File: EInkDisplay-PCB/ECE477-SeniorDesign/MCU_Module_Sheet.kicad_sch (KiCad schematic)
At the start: 26 parts, among them J7 Conn_01x05, SW1 SW_Push_Dual_x2, U3 STM32L496ZGTxP

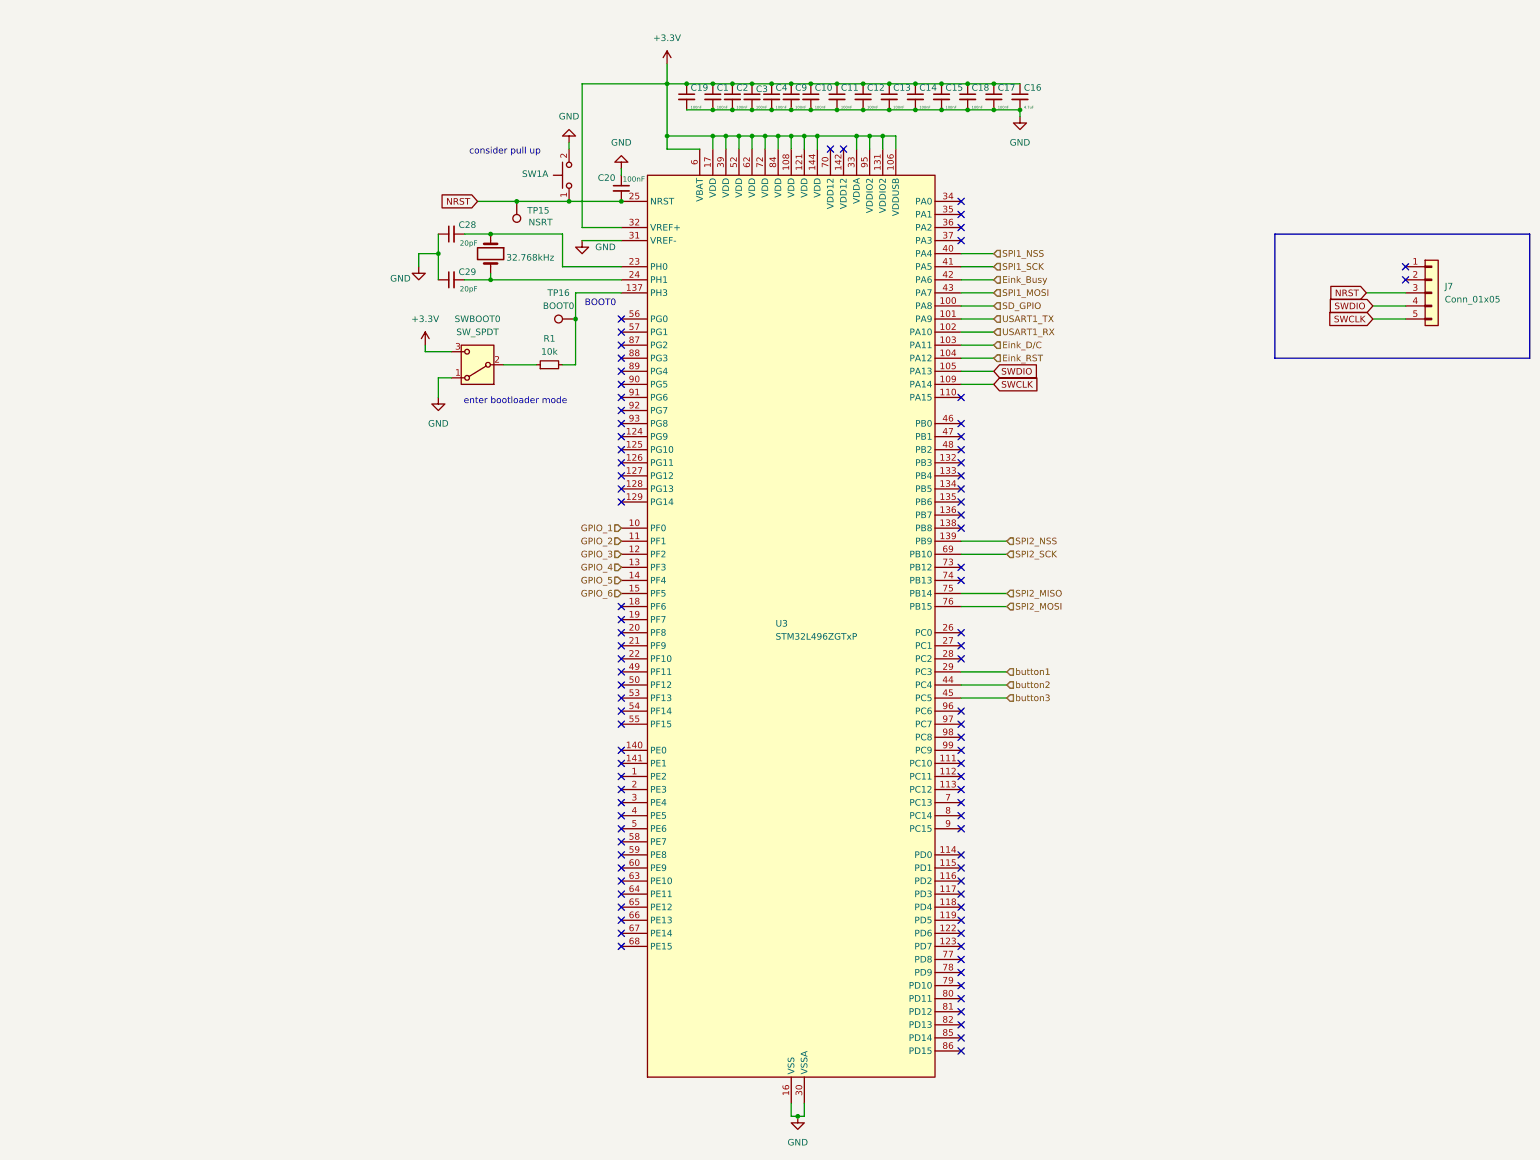
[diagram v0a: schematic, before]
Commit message: Lotta changes
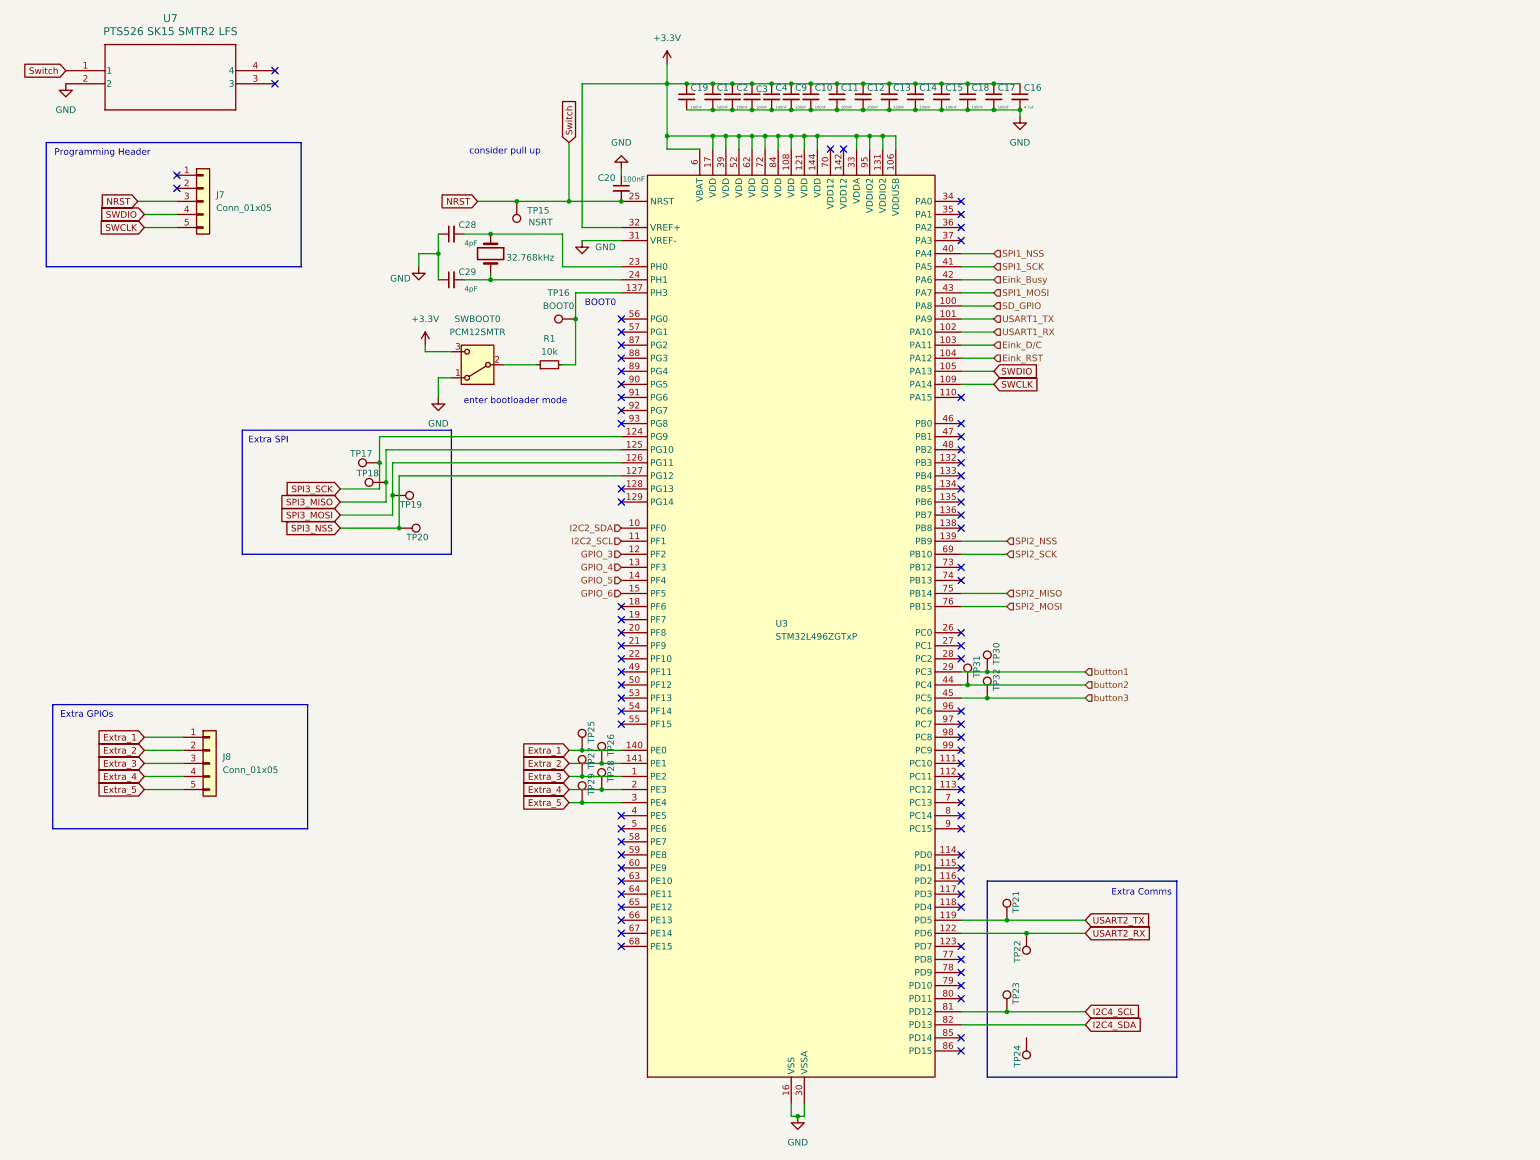
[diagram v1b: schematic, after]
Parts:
- removed SW1: SW_Push_Dual_x2, symbol Switch:SW_Push_Dual_x2
- added J8: Conn_01x05, symbol Connector_Generic:Conn_01x05
- added TP17, TP18, TP19, TP20, TP21, TP22, TP23, TP24, TP25, TP26, TP27, TP28, TP29, TP30, TP31, TP32: ~, symbol Connector:TestPoint
- added U7: PTS526 SK15 SMTR2 LFS, PCB_Lib:PTS256, symbol EinkComponentLibrary:PTS526_SK15_SMTR2_LFS
- C1, C10, C11, C12, C13, C14, C15, C16, C17, C18, C2, C20, C3, C4, C9: footprint (none) -> Capacitor_SMD:C_0805_2012Metric_Pad1.18x1.45mm_HandSolder
- C28, C29: value 20pF -> 4pF; footprint (none) -> Capacitor_SMD:C_0805_2012Metric_Pad1.18x1.45mm_HandSolder
- SWBOOT0: value SW_SPDT -> PCM12SMTR; footprint (none) -> PCB_Lib:PCM12SMTR_CNK
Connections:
- net GND: now also U7.2
- net NRST: now also U7.1
- net button1: now also TP30.1
- net button2: now also TP31.1
- net button3: now also TP32.1
- net Extra_3: now reaches U3.1 (PE2)
- net Extra_3: now also J8.3 (Pin_3), TP27.1
- net USART2_TX: now reaches U3.119 (PD5)
- net USART2_TX: now also TP21.1
- net USART2_RX: now reaches U3.122 (PD6)
- net USART2_RX: now also TP22.1
- net SPI3_SCK: now reaches U3.124 (PG9)
- net SPI3_SCK: now also TP17.1
- net SPI3_MISO: now reaches U3.125 (PG10)
- net SPI3_MISO: now also TP18.1
- net SPI3_MOSI: now reaches U3.126 (PG11)
- net SPI3_MOSI: now also TP19.1
- net SPI3_NSS: now reaches U3.127 (PG12)
- net SPI3_NSS: now also TP20.1
- net Extra_1: now reaches U3.140 (PE0)
- net Extra_1: now also J8.1 (Pin_1), TP25.1
- net Extra_2: now reaches U3.141 (PE1)
- net Extra_2: now also J8.2 (Pin_2), TP26.1
- net Extra_4: now reaches U3.2 (PE3)
- net Extra_4: now also J8.4 (Pin_4), TP28.1
- net Extra_5: now reaches U3.3 (PE4)
- net Extra_5: now also J8.5 (Pin_5), TP29.1
- net I2C4_SCL: now reaches U3.81 (PD12)
- net I2C4_SCL: now also TP23.1
- net I2C4_SDA: now reaches U3.82 (PD13)
- net GPIO_1 renamed I2C2_SDA
- net GPIO_2 renamed I2C2_SCL
- no-connect marks 90 -> 79
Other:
- note added: "Extra Comms"
- note added: "Extra GPIOs"
- note added: "Extra SPI"
- note added: "Programming Header"
- moved on the sheet: J7
